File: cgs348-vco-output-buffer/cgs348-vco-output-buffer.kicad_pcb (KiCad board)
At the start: 2 copper layers, 50.3 x 50.8 mm, 27 parts, among them J9 Power, U1 TL074

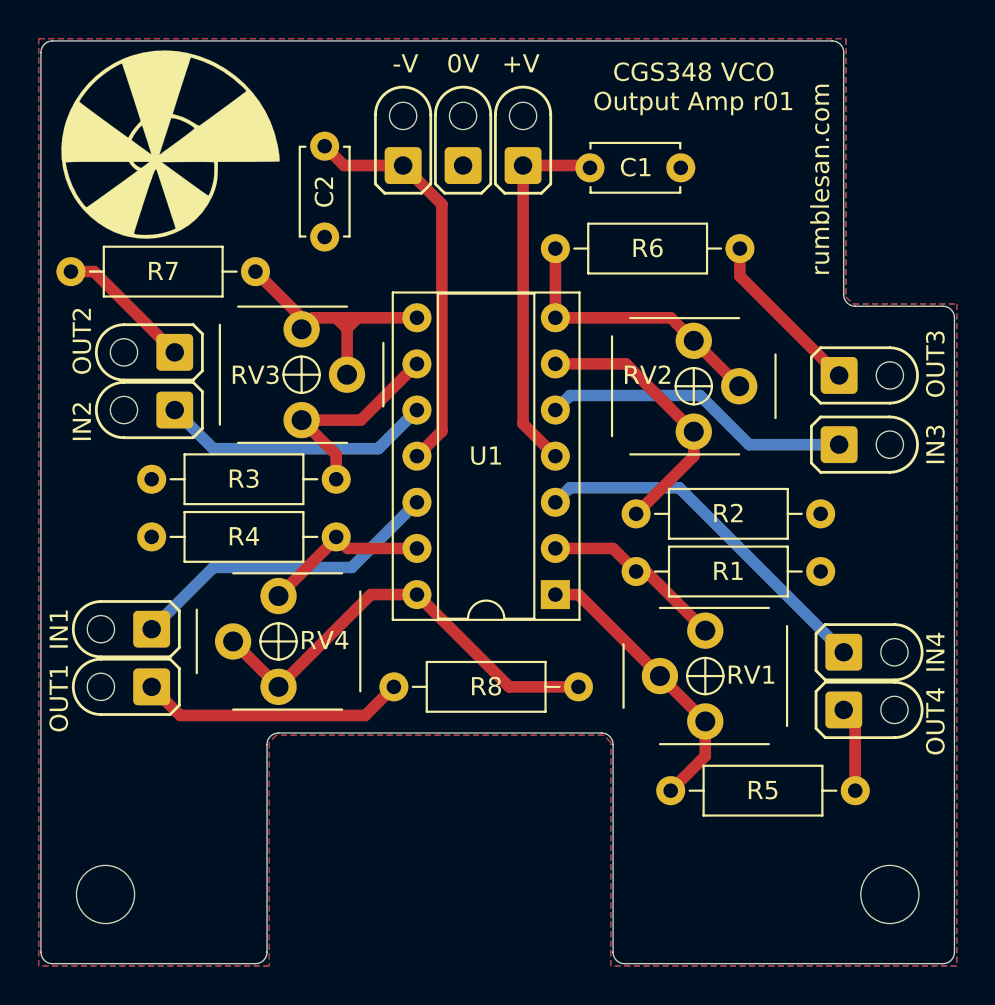
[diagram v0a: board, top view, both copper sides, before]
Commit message: Updating ordered boards
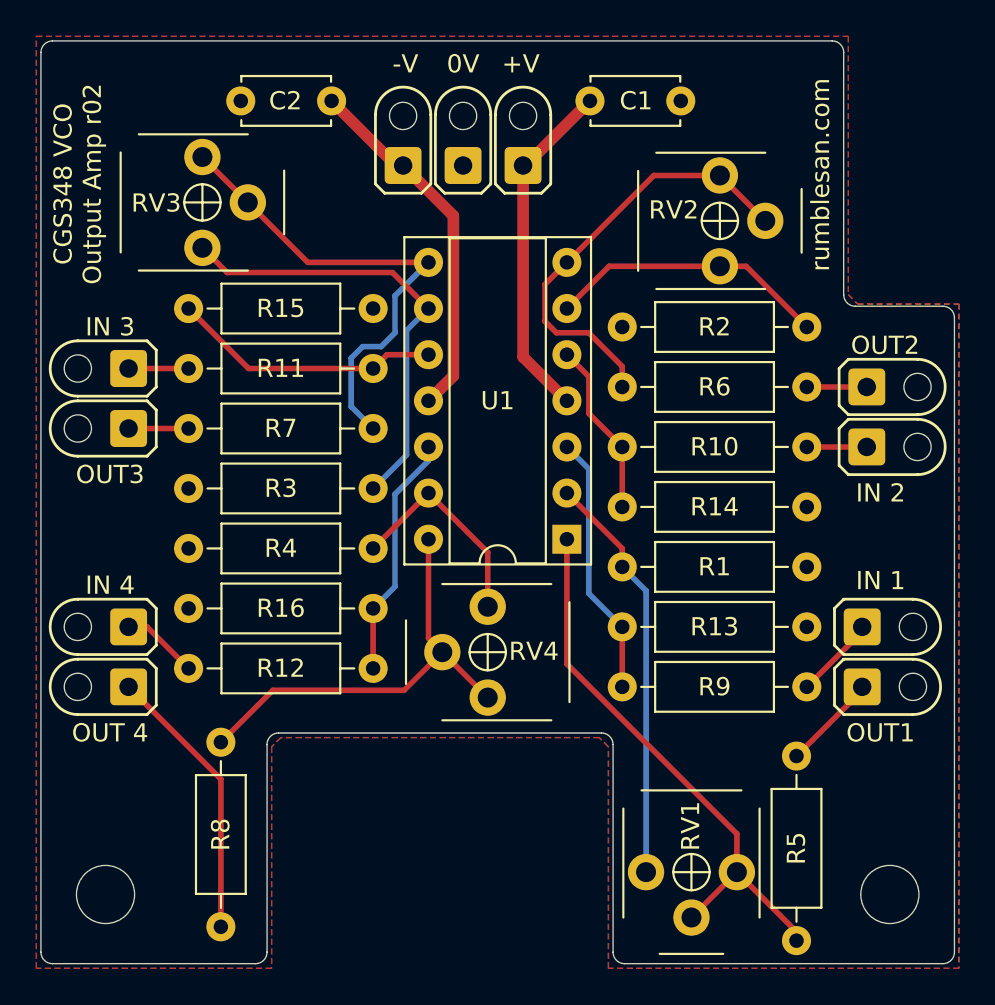
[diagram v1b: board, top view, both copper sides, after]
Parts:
- removed H3: Logo_Ammonite-simple, rumblesan-footprints:Logo_Ammonite-simple_10.4mmx12.0mm
- added R10: 47k, rumblesan-footprints:Resistor_THT_L6.3mm_D2.5mm_P10.16mm_Horizontal, F.Cu at (131.3, 124.0)
- added R11: 47k, rumblesan-footprints:Resistor_THT_L6.3mm_D2.5mm_P10.16mm_Horizontal, F.Cu at (97.3, 119.6)
- added R12: 47k, rumblesan-footprints:Resistor_THT_L6.3mm_D2.5mm_P10.16mm_Horizontal, F.Cu at (97.3, 136.1)
- added R13: 47k, rumblesan-footprints:Resistor_THT_L6.3mm_D2.5mm_P10.16mm_Horizontal, F.Cu at (121.2, 133.9)
- added R14: 47k, rumblesan-footprints:Resistor_THT_L6.3mm_D2.5mm_P10.16mm_Horizontal, F.Cu at (121.2, 127.3)
- added R15: 47k, rumblesan-footprints:Resistor_THT_L6.3mm_D2.5mm_P10.16mm_Horizontal, F.Cu at (97.3, 116.3)
- added R16: 47k, rumblesan-footprints:Resistor_THT_L6.3mm_D2.5mm_P10.16mm_Horizontal, F.Cu at (107.4, 132.8)
- added R9: 47k, rumblesan-footprints:Resistor_THT_L6.3mm_D2.5mm_P10.16mm_Horizontal, F.Cu at (131.3, 137.2)
- moved R8 16.3 mm to (99.1, 150.4), turned to 90 degrees
- moved R2 13.9 mm to (131.3, 117.3), turned to 180 degrees
- moved RV4 11.5 mm to (113.8, 135.2)
- moved RV3 10.9 mm to (98.0, 110.5)
- moved RV1 10.8 mm to (125.0, 147.4), turned to 180 degrees
- moved R7 10.8 mm to (97.3, 122.9)
- moved RV2 9.22 mm to (126.5, 111.5)
- moved C2 8.80 mm to (100.2, 104.9), turned to 0 degrees
- moved R6 8.46 mm to (131.3, 120.7)
- moved J7 4.90 mm to (94.0, 122.9)
- moved R5 3.75 mm to (130.8, 141.0), turned to 270 degrees
- moved C1 3.68 mm to (119.4, 104.9)
- moved J3 3.42 mm to (94.0, 119.6)
- moved U1 3.11 mm to (118.1, 129.0)
- moved R4 2.13 mm to (107.4, 129.5)
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- renumbered IN4 to J1, IN3 to J2, IN2 to J3, IN1 to J4, OUT4 to J5, OUT3 to J6, OUT2 to J7, OUT1 to J8
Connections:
- U1 pad 10: Net-(J3-Pad1) -> Net-(R11-Pad2)
- U1 pad 12: Net-(J4-Pad1) -> Net-(R12-Pad2)
- U1 pad 3: Net-(J1-Pad1) -> Net-(R13-Pad1)
- U1 pad 5: Net-(J2-Pad1) -> Net-(R10-Pad2)
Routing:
- net Net-(J1-Pad1): track 20.0 -> 4.56 mm
- net Net-(R5-Pad2): track 15.7 -> 30.9 mm
- net Net-(R11-Pad2): track 0.00 -> 14.9 mm
- net Net-(R13-Pad1): track 0.00 -> 14.5 mm
- net Net-(J2-Pad1): track 17.1 -> 3.30 mm
- net Net-(R12-Pad2): track 0.00 -> 13.5 mm
- net Net-(R3-Pad1): track 11.7 -> 25.0 mm
- net Net-(J4-Pad1): track 17.5 -> 4.25 mm
- net Net-(R1-Pad1): track 10.1 -> 22.7 mm
- net Net-(J3-Pad1): track 15.1 -> 3.30 mm
- net Net-(R7-Pad2): track 15.8 -> 26.9 mm
- net Net-(R10-Pad2): track 0.00 -> 9.64 mm
- net Net-(R6-Pad2): track 15.5 -> 24.1 mm
- net Net-(J6-Pad1): track 9.25 -> 3.30 mm
- net Net-(J7-Pad1): track 7.56 -> 3.30 mm
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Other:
- rule pad_to_mask_clearance: 0.0508 -> 0
- board text added: "CGS348 VCO Output Amp r02"
- board text added: "IN 1"
- board text added: "IN 2"
- board text added: "IN 3"
- board text added: "IN 4"
- board text added: "OUT 4"
- board text added: "OUT1"
- board text added: "OUT2"
- board text added: "OUT3"
- board text removed: "CGS348 VCO Output Amp r01"
